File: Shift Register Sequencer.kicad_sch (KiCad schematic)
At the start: 105 parts, among them J1 Gate IN, J10 Step 4, J11 Step C, J12 Step 5, J13 Step F, J14 Step 0-F, J2 Step 0, J3 Step 6, J4 Step 1, J5 Step 7, J6 Step 2, J7 Step 8, J8 Step 3, J9 Step A, Q1 2N3904, Q2 2N3904, SW1 oneShot/continous, SW2 oneShot/continous, U1 4070, U2 SN74HC595N, U3 SN74HC595N, U4 TL072, U5 CD4050, U6 CD4050, U7 TL072

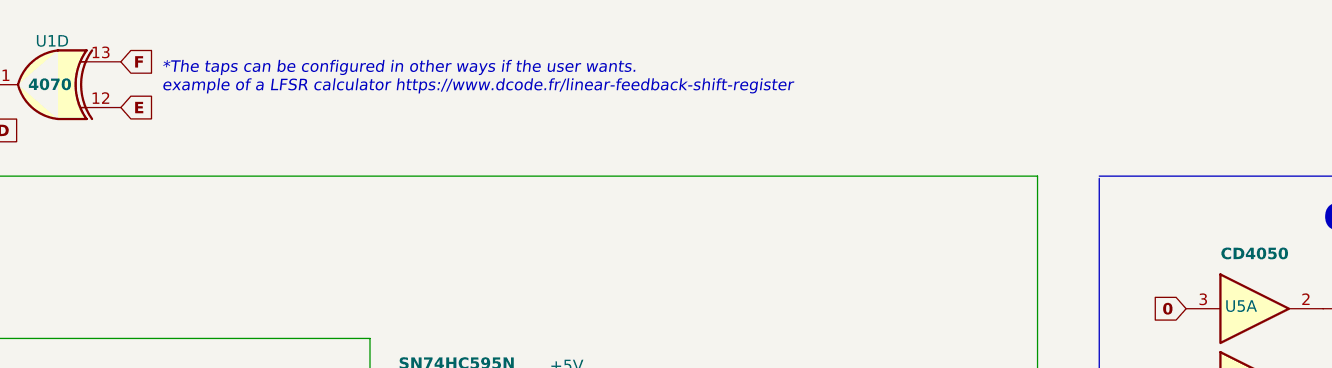
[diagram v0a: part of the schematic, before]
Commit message: Update
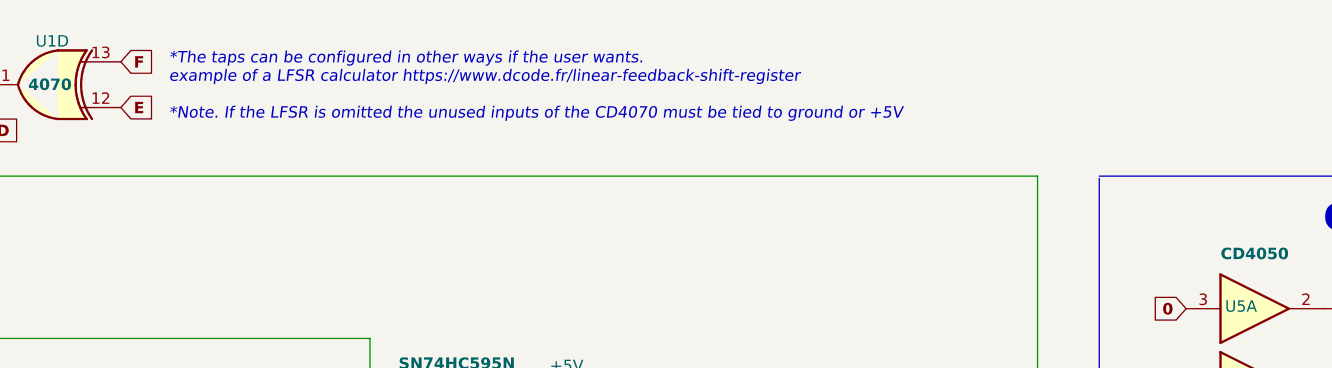
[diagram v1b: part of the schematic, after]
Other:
- note added: "*The taps can be configured in other ways if the user wants. example of a LFSR calculator https://www.dcode.fr/linear-feedback-shift-register *Note. If the LFSR is omitted the unused inputs of the CD4070 must be tied to ground or +5V"
- note removed: "*The taps can be configured in other ways if the user wants. example of a LFSR calculator https://www.dcode.fr/linear-feedback-shift-register"
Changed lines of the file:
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@@
     (effects (font (size 1.27 1.27) (thickness 0.254) bold) (justify left bottom))
   )
-  (text "*The taps can be configured in other ways if the user wants.\nexample of a LFSR calculator https://www.dcode.fr/linear-feedback-shift-register"
-    (at 191.008 27.178 0)
+  (text "*The taps can be configured in other ways if the user wants.\nexample of a LFSR calculator https://www.dcode.fr/linear-feedback-shift-register\n\n*Note. If the LFSR is omitted the unused inputs of the CD4070 must be tied to ground or +5V "
+    (at 191.77 30.226 0)
     (effects (font (size 1.27 1.27) italic) (justify left bottom))
   )
